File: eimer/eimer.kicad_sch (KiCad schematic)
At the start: 21 parts, among them J2 USB_C_Receptacle_USB2.0_14P, U1 RP2040, U2 NCP1117-3.3_SOT223

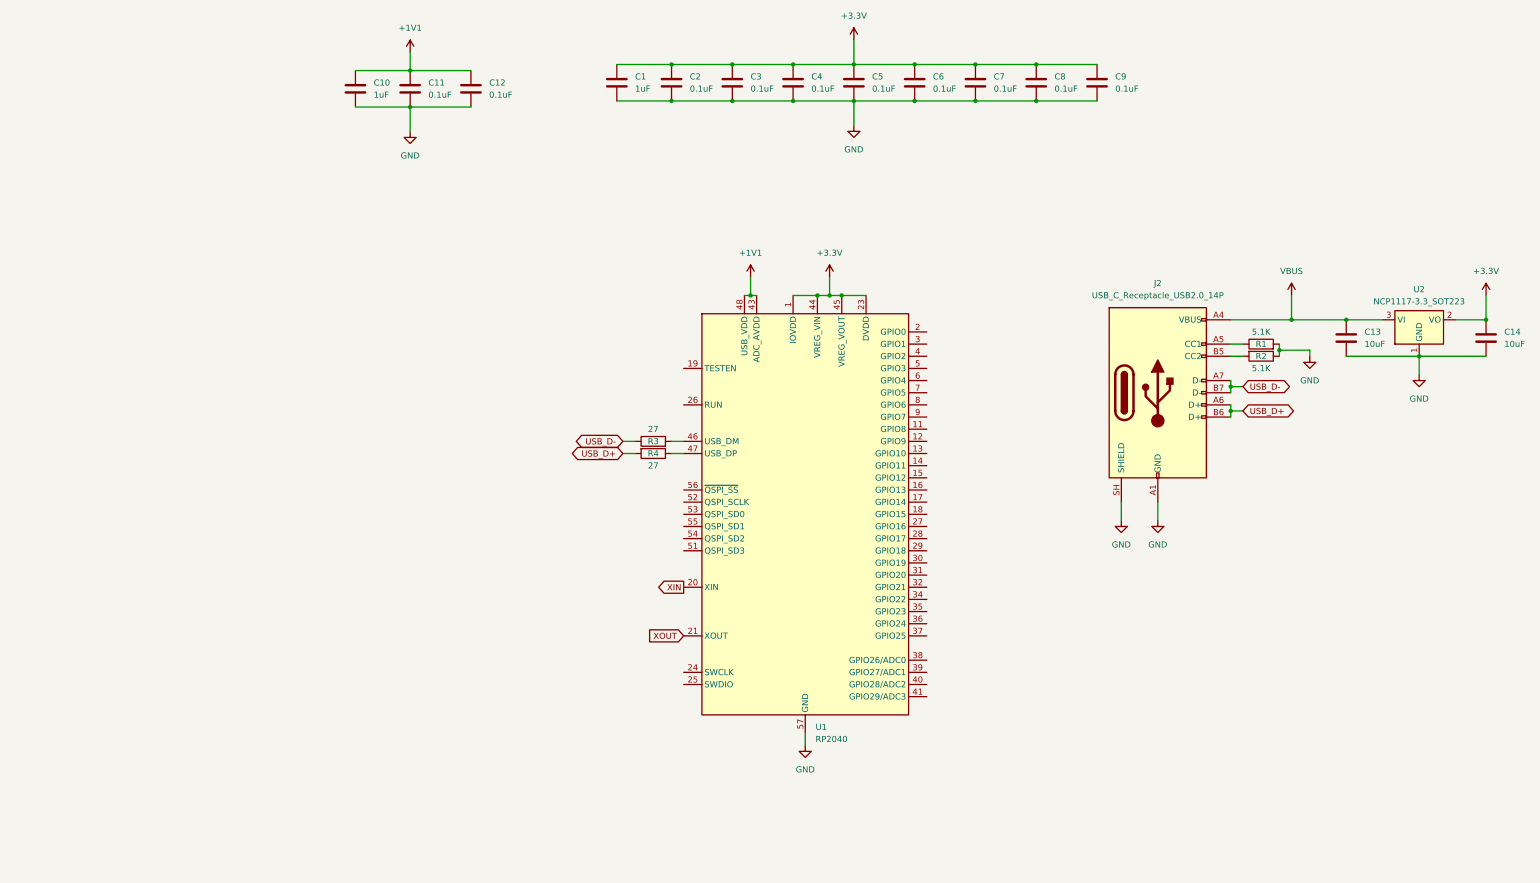
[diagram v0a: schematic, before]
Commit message: more work on schematic
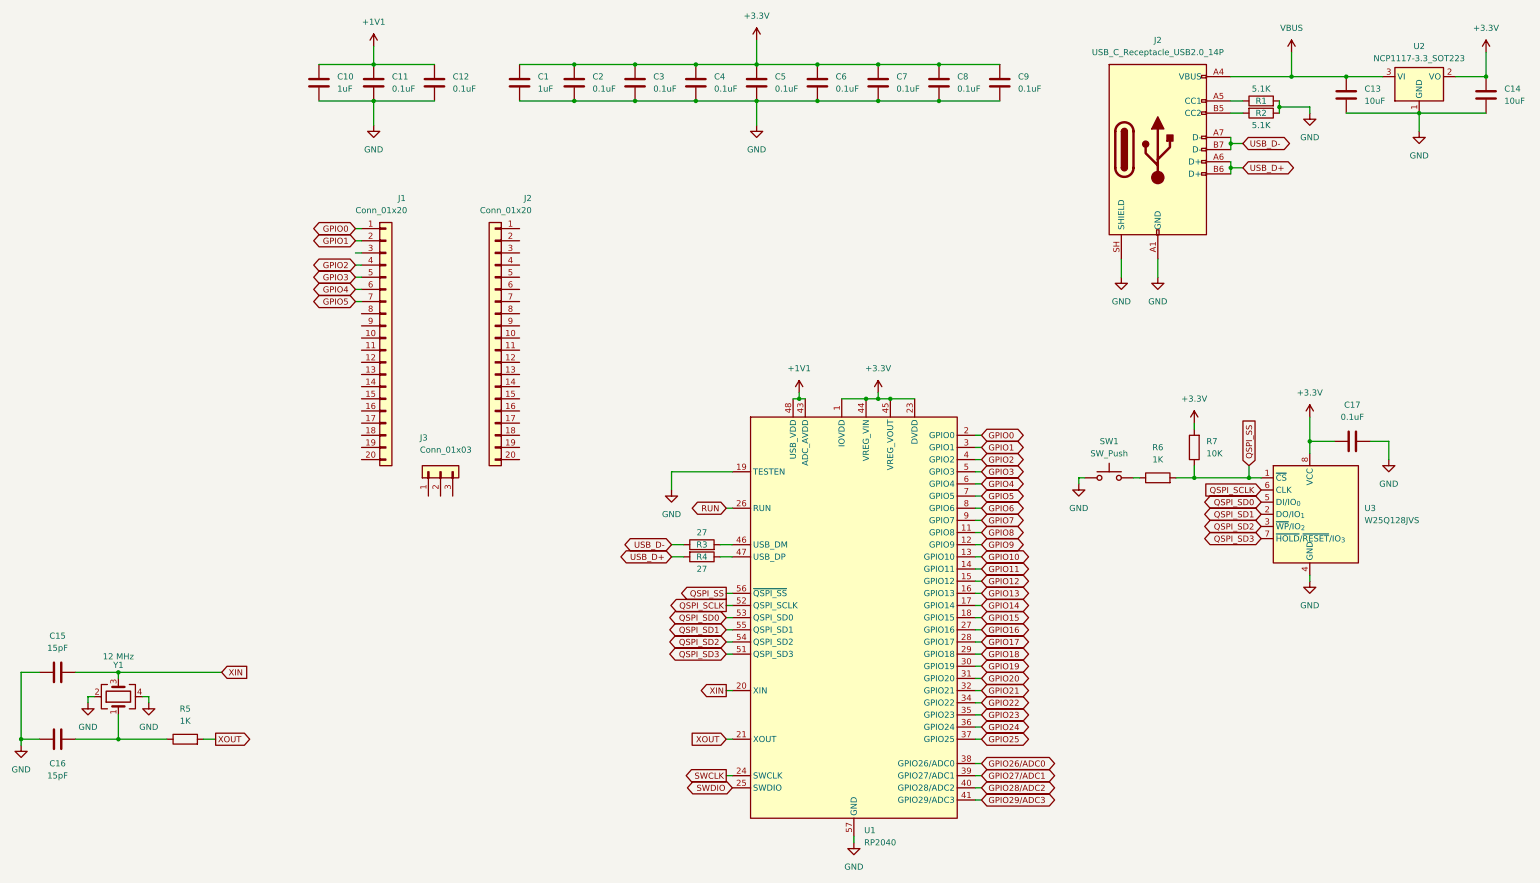
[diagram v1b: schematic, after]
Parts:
- added C15, C16: 15pF, symbol Device:C
- added C17: 0.1uF, symbol Device:C
- added J1: Conn_01x20, symbol Connector_Generic:Conn_01x20
- added J2: Conn_01x20, Connector_PinHeader_2.54mm:PinHeader_1x20_P2.54mm_Vertical, symbol Connector_Generic:Conn_01x20
- added J3: Conn_01x03, Connector_PinHeader_2.54mm:PinHeader_1x03_P2.54mm_Vertical, symbol Connector_Generic:Conn_01x03
- added R5, R6: 1K, symbol Device:R
- added R7: 10K, symbol Device:R
- added SW1: SW_Push, symbol Switch:SW_Push
- added U3: W25Q128JVS, Package_SO:SOIC-8_5.3x5.3mm_P1.27mm, symbol Memory_Flash:W25Q128JVS
- added Y1: 12 MHz, Crystal:Crystal_SMD_3225-4Pin_3.2x2.5mm, symbol Device:Crystal_GND24
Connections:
- net +3.3V: now also C17.1, R7.2, U3.8 (VCC)
- net GND: now also U1.19 (TESTEN), C15.1, C16.2, C17.2, SW1.1, U3.4 (GND), Y1.2, Y1.4
- net XIN: now also C15.2, Y1.3
- net XOUT: now also R5.2
- net GPIO8: now reaches U1.11 (GPIO8)
- net GPIO9: now reaches U1.12 (GPIO9)
- net GPIO10: now reaches U1.13 (GPIO10)
- net GPIO11: now reaches U1.14 (GPIO11)
- net GPIO12: now reaches U1.15 (GPIO12)
- net GPIO13: now reaches U1.16 (GPIO13)
- net GPIO14: now reaches U1.17 (GPIO14)
- net GPIO15: now reaches U1.18 (GPIO15)
- net GPIO0: now reaches U1.2 (GPIO0)
- net GPIO0: now also J1.1 (Pin_1)
- net SWCLK: now reaches U1.24 (SWCLK)
- net SWDIO: now reaches U1.25 (SWDIO)
- net RUN: now reaches U1.26 (RUN)
- net GPIO16: now reaches U1.27 (GPIO16)
- net GPIO17: now reaches U1.28 (GPIO17)
- net GPIO18: now reaches U1.29 (GPIO18)
- net GPIO1: now reaches U1.3 (GPIO1)
- net GPIO1: now also J1.2 (Pin_2)
- net GPIO19: now reaches U1.30 (GPIO19)
- net GPIO20: now reaches U1.31 (GPIO20)
- net GPIO21: now reaches U1.32 (GPIO21)
- net GPIO22: now reaches U1.34 (GPIO22)
- net GPIO23: now reaches U1.35 (GPIO23)
- net GPIO24: now reaches U1.36 (GPIO24)
- net GPIO25: now reaches U1.37 (GPIO25)
- net GPIO26/ADC0: now reaches U1.38 (GPIO26/ADC0)
- net GPIO27/ADC1: now reaches U1.39 (GPIO27/ADC1)
- net GPIO2: now reaches U1.4 (GPIO2)
- net GPIO2: now also J1.4 (Pin_4)
- net GPIO28/ADC2: now reaches U1.40 (GPIO28/ADC2)
- net GPIO29/ADC3: now reaches U1.41 (GPIO29/ADC3)
- net GPIO3: now reaches U1.5 (GPIO3)
- net GPIO3: now also J1.5 (Pin_5)
- net QSPI_SD3: now reaches U1.51 (QSPI_SD3)
- net QSPI_SD3: now also U3.7 (~{HOLD}/~{RESET}/IO_{3})
- net QSPI_SCLK: now reaches U1.52 (QSPI_SCLK)
- net QSPI_SCLK: now also U3.6 (CLK)
- net QSPI_SD0: now reaches U1.53 (QSPI_SD0)
- net QSPI_SD0: now also U3.5 (DI/IO_{0})
- net QSPI_SD2: now reaches U1.54 (QSPI_SD2)
- net QSPI_SD2: now also U3.3 (~{WP}/IO_{2})
- net QSPI_SD1: now reaches U1.55 (QSPI_SD1)
- net QSPI_SD1: now also U3.2 (DO/IO_{1})
- net QSPI_SS: now reaches U1.56 (~{QSPI_SS})
- net QSPI_SS: now also R6.2, R7.1, U3.1 (~{CS})
- net GPIO4: now reaches U1.6 (GPIO4)
- net GPIO4: now also J1.6 (Pin_6)
- net GPIO5: now reaches U1.7 (GPIO5)
- net GPIO5: now also J1.7 (Pin_7)
- net GPIO6: now reaches U1.8 (GPIO6)
- net GPIO7: now reaches U1.9 (GPIO7)
- new net: R6.1, SW1.2
- new net: C16.1, R5.1, Y1.1
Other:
- moved on the sheet: C1, C10, C11, C12, C13, C14, C2, C3, C4, C5, C6, C7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
